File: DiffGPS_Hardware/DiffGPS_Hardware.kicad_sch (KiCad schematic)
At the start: 15 parts, among them U1 Raspberry_Pi, U2 OKI

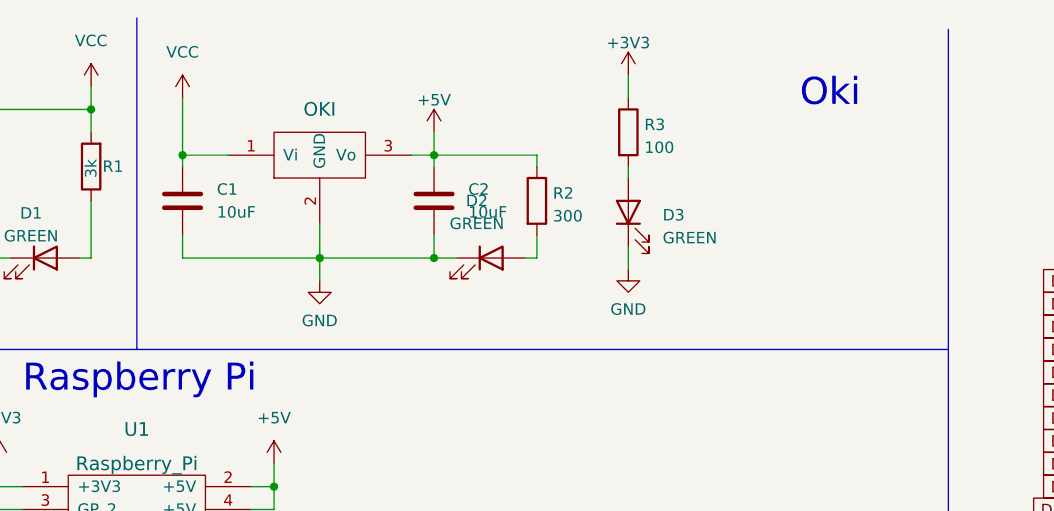
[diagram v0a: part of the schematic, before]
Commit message: tried to make buck converter
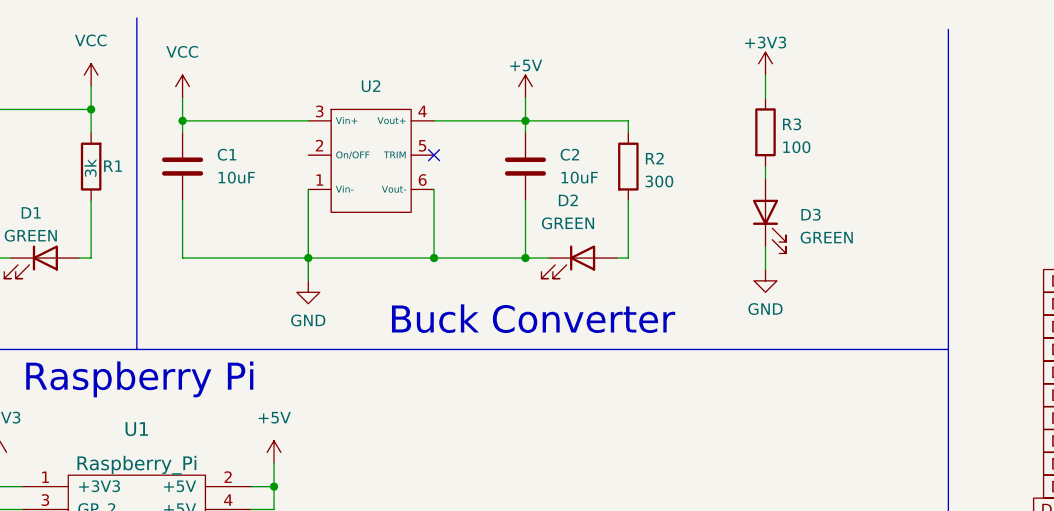
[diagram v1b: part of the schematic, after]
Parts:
- removed U2: OKI, MRDT_Devices:OKI_Horizontal, symbol MRDT_Devices:OKI
- added U2: ~, symbol SHHD003A0A:SHHD003A0A
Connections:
- net +5V: now also U2.4 (Vout+)
- net GND: now also U2.1 (Vin-), U2.6 (Vout-)
- net VCC: now also U2.3 (Vin+)
- no-connect marks 15 -> 16
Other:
- note added: "Buck Converter"
- note removed: "Oki"
- moved on the sheet: C1, C2, D2, D3, R2, R3
